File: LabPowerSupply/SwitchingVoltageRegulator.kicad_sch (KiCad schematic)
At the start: 14 parts

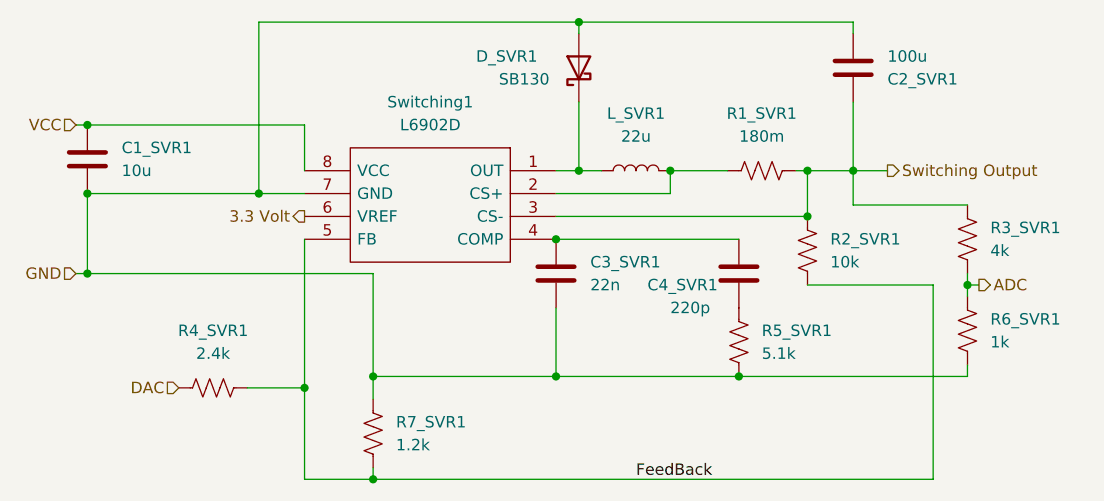
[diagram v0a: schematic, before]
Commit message: another commit
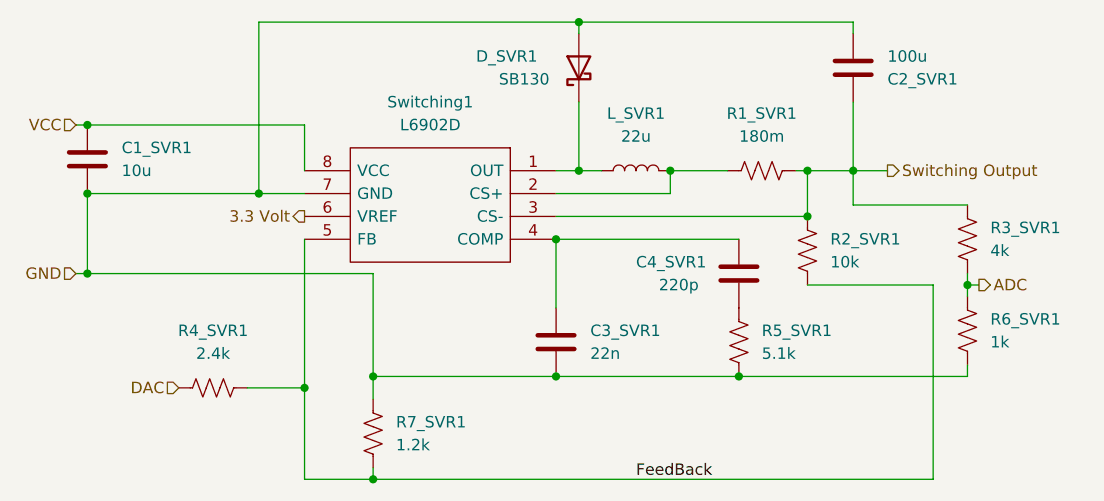
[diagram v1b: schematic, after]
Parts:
- C3_SVR1: footprint Capacitor_THT:C_Disc_D7.0mm_W2.5mm_P5.00mm -> Capacitor_THT:C_Disc_D7.5mm_W2.5mm_P5.00mm
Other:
- moved on the sheet: C3_SVR1
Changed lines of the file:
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@@
+    (stroke (width 0) (type default) (color 0 0 0 0))
+  )
+  (wire (pts (xy 138.43 107.95) (xy 138.43 100.33))
     (stroke (width 0) (type default) (color 0 0 0 0))
   )
@@
   )
   (wire (pts (xy 118.11 125.73) (xy 118.11 127))
-    (stroke (width 0) (type default) (color 0 0 0 0))
-  )
-  (wire (pts (xy 138.43 107.95) (xy 138.43 115.57))
     (stroke (width 0) (type default) (color 0 0 0 0))
   )
@@
     (pin "2")
   )
-  (symbol (lib_id "Device:C") (at 138.43 104.14 0) (unit 1)
-    (in_bom yes) (on_board yes) (fields_autoplaced)
-    (property "Reference" "C3_SVR1" (id 0) (at 142.24 102.8699 0)
-      (effects (font (size 1.27 1.27)) (justify left))
-    )
-    (property "Value" "22n" (id 1) (at 142.24 105.4099 0)
-      (effects (font (size 1.27 1.27)) (justify left))
-    )
-    (property "Footprint" "Capacitor_THT:C_Disc_D7.0mm_W2.5mm_P5.00mm" (id 2) (at 139.3952 107.95 0)
-      (effects (font (size 1.27 1.27)) hide)
-    )
-    (property "Datasheet" "~" (id 3) (at 138.43 104.14 0)
+  (symbol (lib_id "Device:C") (at 138.43 111.76 0) (unit 1)
+    (in_bom yes) (on_board yes) (fields_autoplaced)
+    (property "Reference" "C3_SVR1" (id 0) (at 142.24 110.4899 0)
+      (effects (font (size 1.27 1.27)) (justify left))
+    )
+    (property "Value" "22n" (id 1) (at 142.24 113.0299 0)
+      (effects (font (size 1.27 1.27)) (justify left))
+    )
+    (property "Footprint" "Capacitor_THT:C_Disc_D7.5mm_W2.5mm_P5.00mm" (id 2) (at 139.3952 115.57 0)
+      (effects (font (size 1.27 1.27)) hide)
+    )
+    (property "Datasheet" "~" (id 3) (at 138.43 111.76 0)
       (effects (font (size 1.27 1.27)) hide)
     )
@@
   (symbol (lib_id "Device:C") (at 158.75 104.14 0) (unit 1)
     (in_bom yes) (on_board yes)
-    (property "Reference" "C4_SVR1" (id 0) (at 148.59 105.41 0)
-      (effects (font (size 1.27 1.27)) (justify left))
-    )
-    (property "Value" "220p" (id 1) (at 151.13 107.95 0)
-      (effects (font (size 1.27 1.27)) (justify left))
-    )
+    (property "Reference" "C4_SVR1" (id 0) (at 147.32 102.87 0)
+      (effects (font (size 1.27 1.27)) (justify left))
+    )
+    (property "Value" "220p" (id 1) (at 149.86 105.41 0)
+      (effects (font (size 1.27 1.27)) (justify left))
+    )
